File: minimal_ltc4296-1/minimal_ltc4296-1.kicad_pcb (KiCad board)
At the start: 4 copper layers, 71.1 x 50.8 mm, 44 parts, among them J1 TBP02R1-381-03BE, J2 TBP02R1-381-03BE, J3 TBP02R1-381-03BE, J4 TBP02R1-381-03BE, J5 TBP02R1-381-03BE, J6 TBP02R1-381-02BE, Q1 100.0 V, Q2 100.0 V, Q3 100.0 V, Q4 100.0 V, Q5 100.0 V, Q6 100.0 V, U1 LTC4296AUK-1-PBF

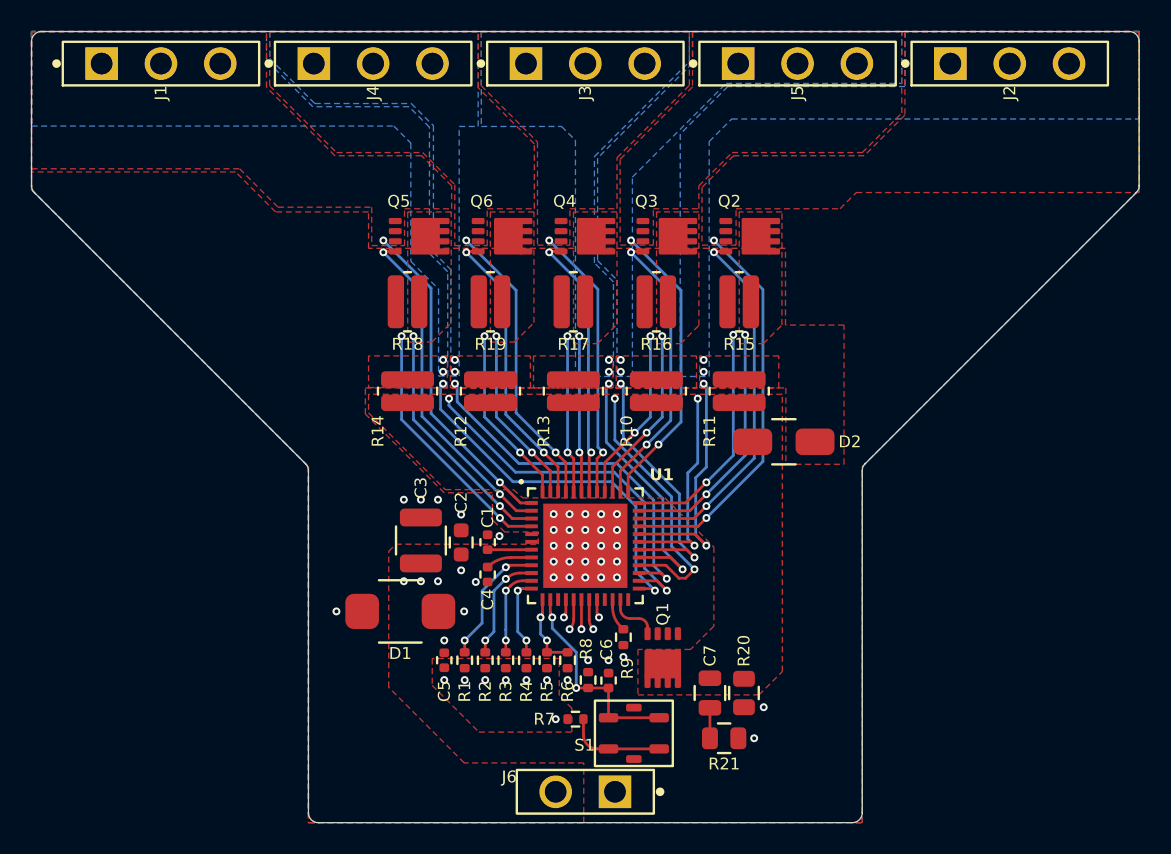
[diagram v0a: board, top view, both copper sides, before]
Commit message: Update KiCad PCB file
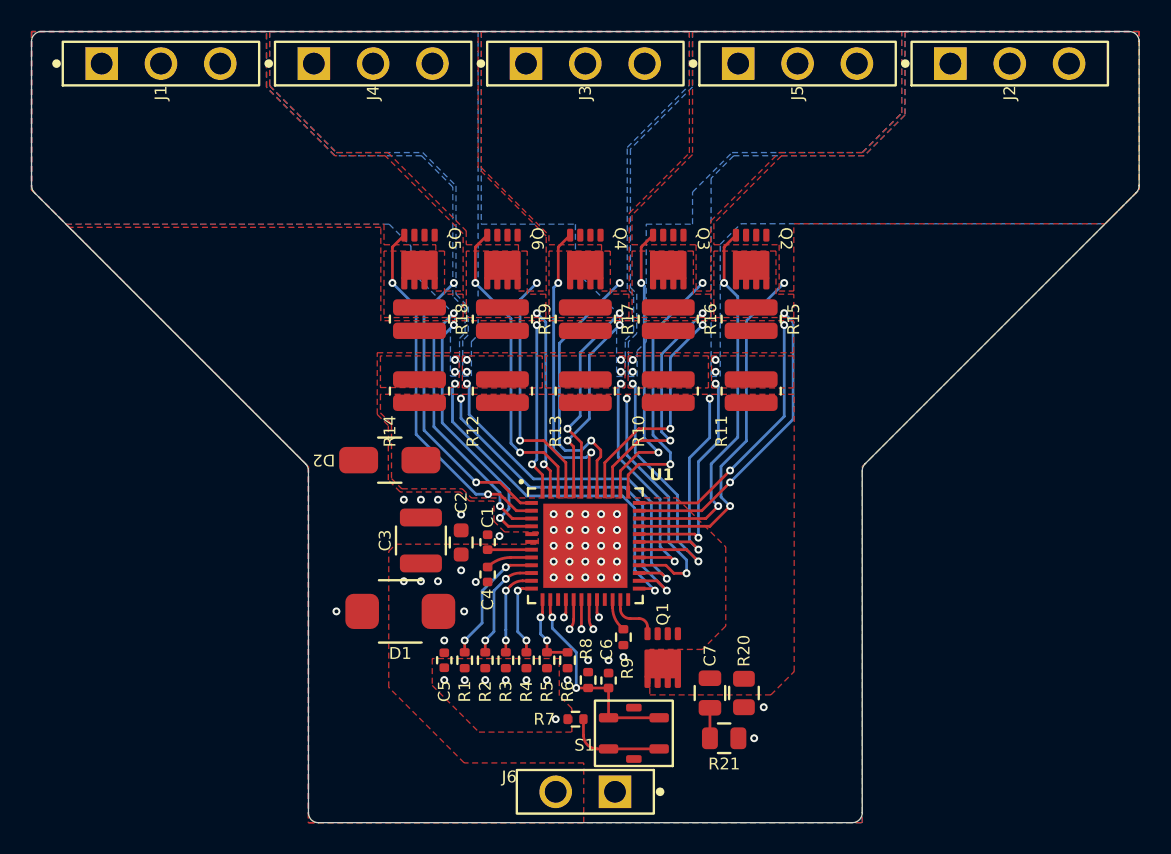
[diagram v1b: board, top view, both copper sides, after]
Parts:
- moved D2 25.3 mm to (137.2, 96.9), turned to 0 degrees
- moved Q3 1.47 mm to (155.0, 84.0), turned to -90 degrees
- moved Q2 1.47 mm to (160.4, 84.0), turned to -90 degrees
- moved Q4 1.47 mm to (149.7, 84.0), turned to -90 degrees
- moved Q5 1.47 mm to (139.1, 84.0), turned to -90 degrees
- moved Q6 1.47 mm to (144.4, 84.0), turned to -90 degrees
- moved R18 1.35 mm to (139.1, 87.8), turned to 90 degrees
- moved R19 1.35 mm to (144.4, 87.8), turned to 90 degrees
- moved R17 1.35 mm to (149.7, 87.8), turned to 90 degrees
- moved R16 1.35 mm to (155.0, 87.8), turned to 90 degrees
- moved R15 1.35 mm to (160.4, 87.8), turned to 90 degrees
- moved R10 0.77 mm to (155.0, 92.4)
- moved R11 0.77 mm to (160.4, 92.4)
- moved R12 0.77 mm to (144.4, 92.4)
- moved R13 0.77 mm to (149.7, 92.4)
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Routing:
- net /PSE: track 64.5 -> 72.4 mm
- net /HSNSM3: track 11.4 -> 15.5 mm
- net /HSNSM4: track 16.0 -> 19.4 mm
- net /HSNSM2: track 10.1 -> 13.2 mm
- net /OUTP1: track 18.8 -> 16.0 mm
- net /OUTP4: track 25.2 -> 22.6 mm
- net /HGATE2: track 17.3 -> 19.5 mm
- net /OUTP0: track 21.2 -> 19.1 mm
- net /OUTM2: track 17.1 -> 15.4 mm
- net /HSNSM0: track 15.6 -> 17.0 mm
- net /OUTP3: track 18.9 -> 17.5 mm
- net /HGATE0: track 21.9 -> 23.2 mm
- net /HGATE1: track 18.6 -> 19.9 mm
- net /OUTM4: track 15.7 -> 14.4 mm
- net /LSNS: track 54.6 -> 54.0 mm
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
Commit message: Update PCB file
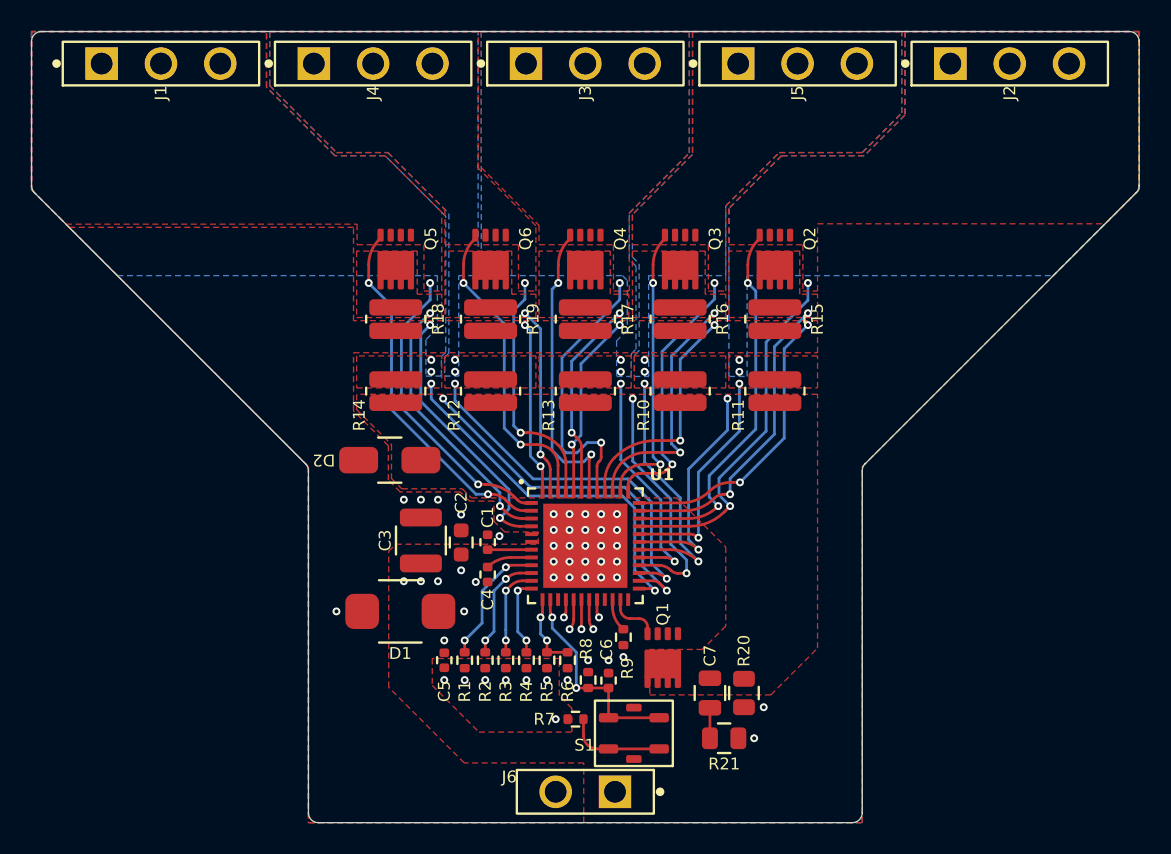
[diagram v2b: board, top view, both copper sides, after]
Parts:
- moved Q2 1.52 mm to (161.9, 84.0)
- moved Q5 1.52 mm to (137.5, 84.0)
- moved R11 1.52 mm to (161.9, 92.4)
- moved R14 1.52 mm to (137.5, 92.4)
- moved R15 1.52 mm to (161.9, 87.8)
- moved R18 1.52 mm to (137.5, 87.8)
- moved Q3 0.76 mm to (155.8, 84.0)
- moved Q6 0.76 mm to (143.6, 84.0)
- moved R10 0.76 mm to (155.8, 92.4)
- moved R12 0.76 mm to (143.6, 92.4)
- moved R16 0.76 mm to (155.8, 87.8)
- moved R19 0.76 mm to (143.6, 87.8)
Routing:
- net /PSE: track 72.4 -> 74.5 mm
- net /HSNSM3: track 15.5 -> 16.3 mm
- net /LSNS: track 54.0 -> 54.6 mm
- net /OUTP4: track 22.6 -> 23.2 mm
- net /HSNSM0: track 17.0 -> 17.6 mm
